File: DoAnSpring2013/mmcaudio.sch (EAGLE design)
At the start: 85 parts, among them IC1 TL082, IC2 TL082, IC3 LM1117, IC4 TL082, IC5 TL082, U1 DAC0808LCN, U2 TEA2025B, X1 HD44780LCD-1602

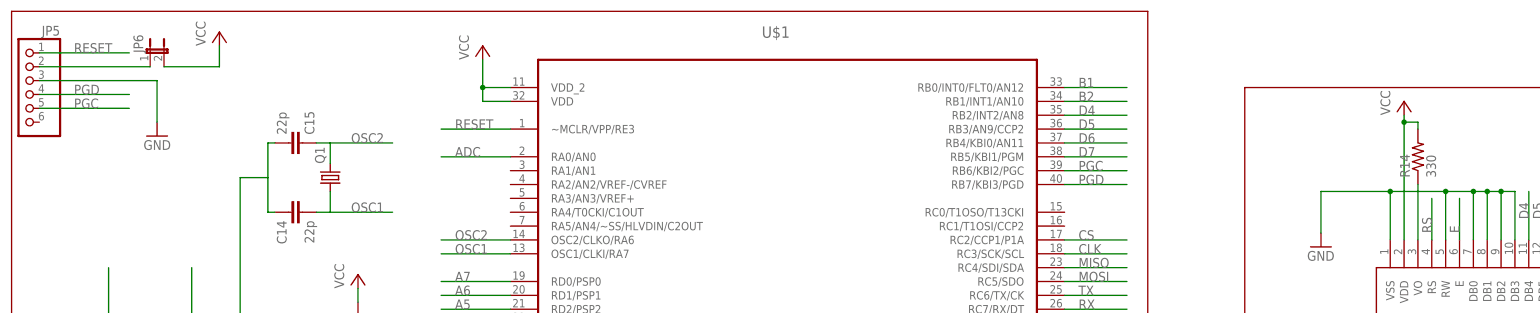
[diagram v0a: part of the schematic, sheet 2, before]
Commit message: routing failed 12:56SA 20131105
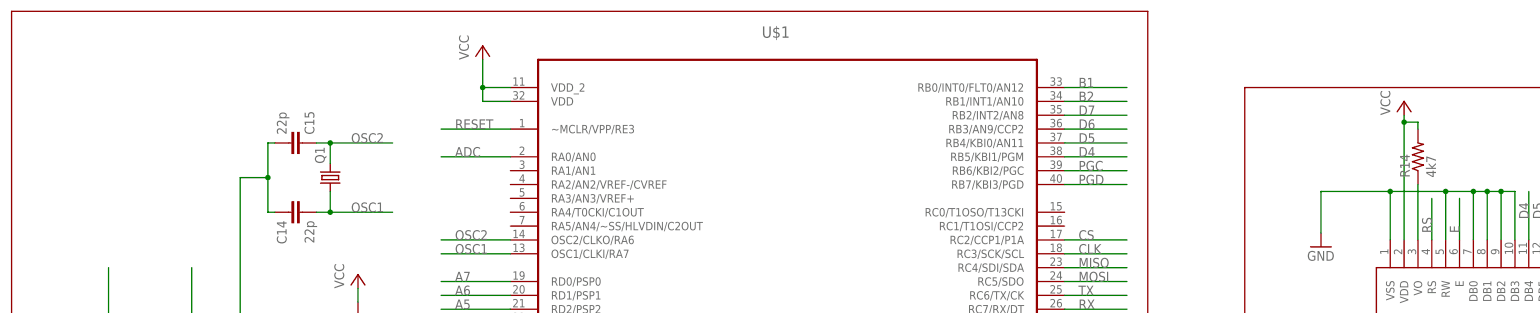
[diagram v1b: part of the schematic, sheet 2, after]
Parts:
- removed JP7: SPEAKER, datle-conn:PINHD-1X20.5"
- removed JP8: (no value), datle-conn:PINHD-1X1
- JP5: value (none) -> SPEAKER; device datle-conn:PINHD-1X6 -> datle-conn:PINHD-1X20.5"
- JP6: device datle-conn:JP1E -> datle-conn:PINHD-1X1
- R14: value 330 -> 4k7
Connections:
- removed net N$42: JP5.2, JP6.1
- net D4: now also U$1.RB5/KBI1/PGM; no longer U$1.RB2/INT2/AN8
- net D5: now also U$1.RB4/KBI0/AN11; no longer U$1.RB3/AN9/CCP2
- net D6: now also U$1.RB3/AN9/CCP2; no longer U$1.RB4/KBI0/AN11
- net D7: now also U$1.RB2/INT2/AN8; no longer U$1.RB5/KBI1/PGM
- net GND: now also JP5.2; no longer JP5.3, JP7.2
- net N$21: now also JP6.1; no longer JP8.1
- net N$25: now also JP5.1; no longer JP7.1
- net PGC: no longer JP5.5
- net PGD: no longer JP5.4
- net RESET: no longer JP5.1
- net VCC: no longer JP6.2
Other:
- moved on the sheet: R23

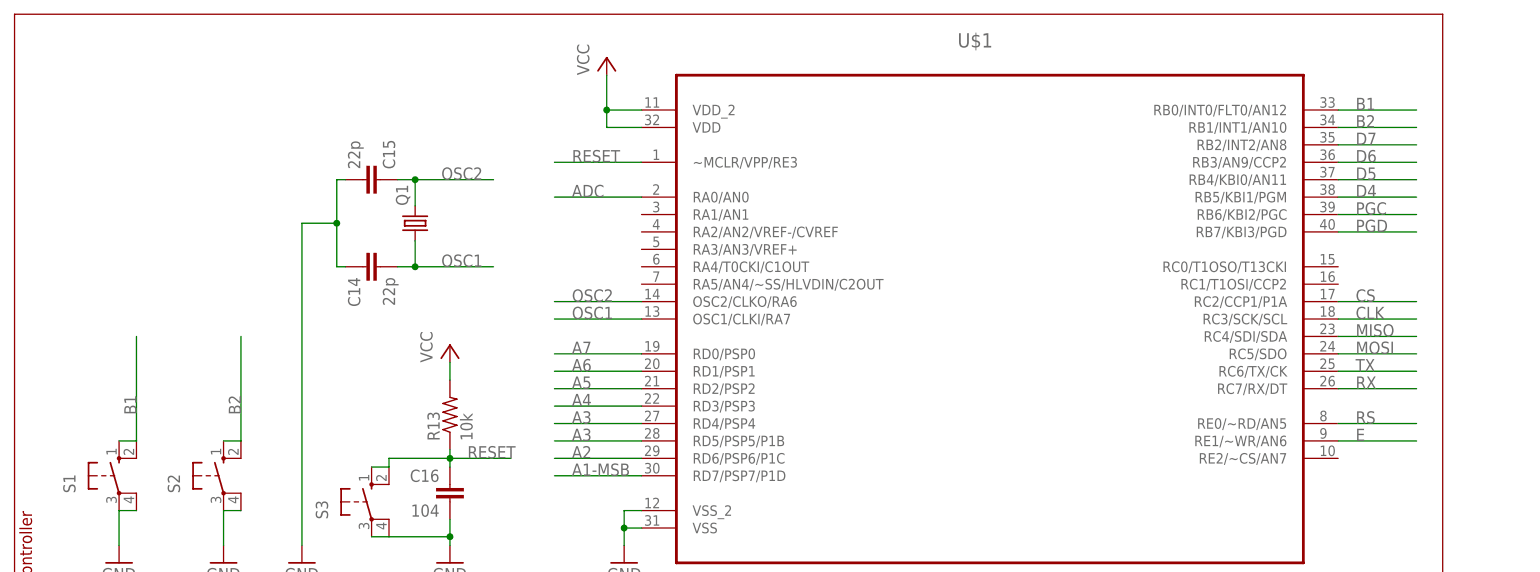
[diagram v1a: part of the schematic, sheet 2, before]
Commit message: route done 1
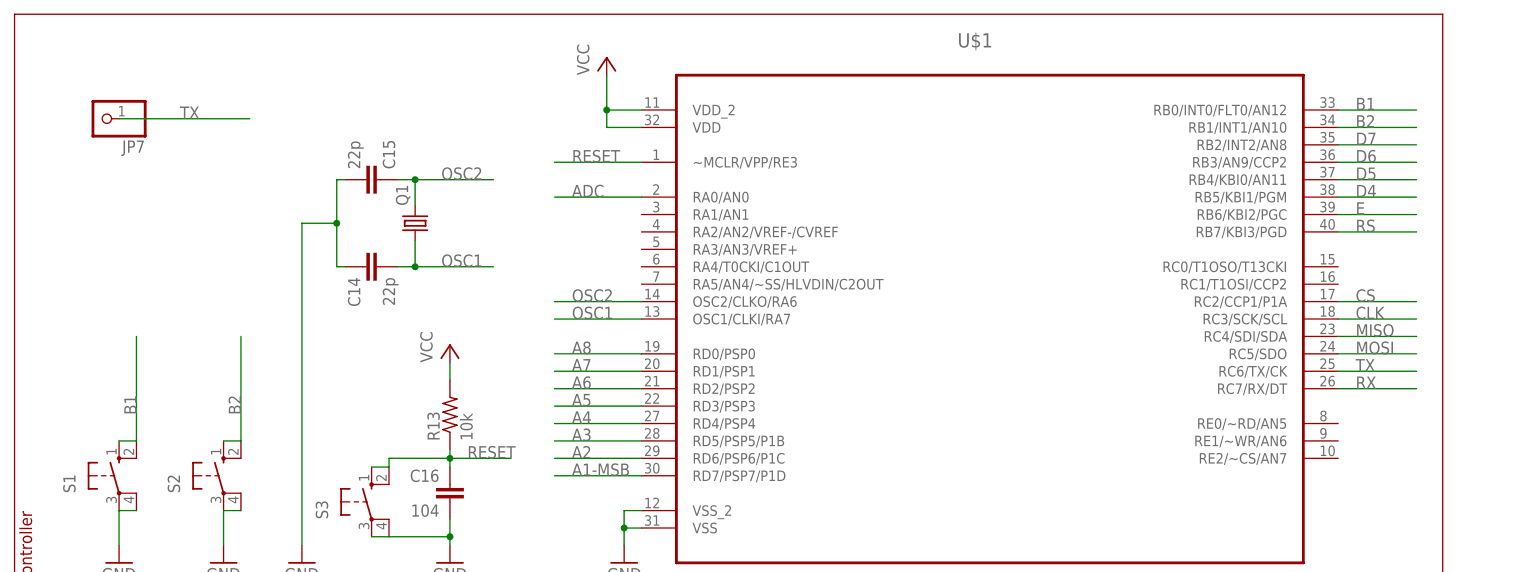
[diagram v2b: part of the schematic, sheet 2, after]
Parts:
- added JP7: (no value), datle-conn:PINHD-1X1
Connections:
- removed net N$35: U$1.RD5/PSP5/P1B
- removed net PGC: U$1.RB6/KBI2/PGC
- removed net PGD: U$1.RB7/KBI3/PGD
- net A3: now also U$1.RD5/PSP5/P1B; no longer U$1.RD4/PSP4
- net A4: now also U$1.RD4/PSP4; no longer U$1.RD3/PSP3
- net A5: now also U$1.RD3/PSP3; no longer U$1.RD2/PSP2
- net A6: now also U$1.RD2/PSP2; no longer U$1.RD1/PSP1
- net A7: now also U$1.RD1/PSP1; no longer U$1.RD0/PSP0
- net A8: now also U$1.RD0/PSP0
- net E: now also U$1.RB6/KBI2/PGC; no longer U$1.RE1/~WR/AN6
- net RS: now also U$1.RB7/KBI3/PGD; no longer U$1.RE0/~RD/AN5
- net TX: now also JP7.1
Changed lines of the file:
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@@
 <setting verticaltext="up"/>
 </settings>
-<grid distance="0.1" unitdist="inch" unit="inch" style="lines" multiple="1" display="no" altdistance="0.01" altunitdist="inch" altunit="mil"/>
+<grid distance="50" unitdist="mil" unit="mil" style="lines" multiple="1" display="yes" altdistance="0.01" altunitdist="inch" altunit="mil"/>
 <layers>
 <layer number="1" name="Top" color="4" fill="1" visible="no" active="no"/>
@@
 <part name="GND1" library="supply1" deviceset="GND" device=""/>
 <part name="GND19" library="supply1" deviceset="GND" device=""/>
+<part name="JP7" library="datle-conn" deviceset="PINHD-1X1" device=""/>
 </parts>
 <sheets>
@@
 <instance part="GND1" gate="1" x="66.04" y="99.06"/>
 <instance part="GND19" gate="1" x="81.28" y="99.06"/>
+<instance part="JP7" gate="G$1" x="63.5" y="163.83" rot="R180"/>
 </instances>
 <busses>
@@
 </segment>
 <segment>
-<pinref part="U$1" gate="A" pin="RE0/~RD/AN5"/>
-<wire x1="243.84" y1="119.38" x2="255.27" y2="119.38" width="0.1524" layer="91"/>
-<label x="246.38" y="119.38" size="1.778" layer="95"/>
+<pinref part="U$1" gate="A" pin="RB7/KBI3/PGD"/>
+<wire x1="243.84" y1="147.32" x2="255.27" y2="147.32" width="0.1524" layer="91"/>
+<label x="246.38" y="147.32" size="1.778" layer="95"/>
 </segment>
 </net>
@@
 <label x="316.23" y="138.43" size="1.778" layer="95" rot="R90"/>
 </segment>
-<segment>
-<pinref part="U$1" gate="A" pin="RE1/~WR/AN6"/>
-<wire x1="243.84" y1="116.84" x2="255.27" y2="116.84" width="0.1524" layer="91"/>
-<label x="246.38" y="116.84" size="1.778" layer="95"/>
-</segment>
-</net>
-<net name="PGD" class="0">
-<segment>
-<pinref part="U$1" gate="A" pin="RB7/KBI3/PGD"/>
-<wire x1="243.84" y1="147.32" x2="255.27" y2="147.32" width="0.1524" layer="91"/>
-<label x="246.38" y="147.32" size="1.778" layer="95"/>
-</segment>
-</net>
-<net name="PGC" class="0">
 <segment>
 <pinref part="U$1" gate="A" pin="RB6/KBI2/PGC"/>
@@
 <label x="246.38" y="127" size="1.778" layer="95"/>
 </segment>
+<segment>
+<pinref part="JP7" gate="G$1" pin="1"/>
+<wire x1="66.04" y1="163.83" x2="85.09" y2="163.83" width="0.1524" layer="91"/>
+<label x="74.93" y="163.83" size="1.778" layer="95"/>
+</segment>
 </net>
 <net name="RX" class="0">
@@
 </segment>
 </net>
-<net name="A3" class="0">
+<net name="A4" class="0">
 <segment>
 <pinref part="U$1" gate="A" pin="RD4/PSP4"/>
-<wire x1="129.54" y1="119.38" x2="142.24" y2="119.38" width="0.1524" layer="91"/>
-<label x="132.08" y="116.84" size="1.778" layer="95"/>
+<wire x1="142.24" y1="119.38" x2="129.54" y2="119.38" width="0.1524" layer="91"/>
 <label x="132.08" y="119.38" size="1.778" layer="95"/>
 </segment>
 </net>
-<net name="A4" class="0">
+<net name="A5" class="0">
 <segment>
 <pinref part="U$1" gate="A" pin="RD3/PSP3"/>
@@
 </segment>
 </net>
-<net name="A5" class="0">
+<net name="A6" class="0">
 <segment>
 <pinref part="U$1" gate="A" pin="RD2/PSP2"/>
@@
 </segment>
 </net>
-<net name="A6" class="0">
+<net name="A7" class="0">
 <segment>
 <pinref part="U$1" gate="A" pin="RD1/PSP1"/>
@@
 </segment>
 </net>
-<net name="A7" class="0">
-<segment>
-<pinref part="U$1" gate="A" pin="RD0/PSP0"/>
-<wire x1="142.24" y1="129.54" x2="129.54" y2="129.54" width="0.1524" layer="91"/>
-<label x="132.08" y="129.54" size="1.778" layer="95"/>
-</segment>
-</net>
-<net name="N$35" class="0">
+<net name="A3" class="0">
 <segment>
 <pinref part="U$1" gate="A" pin="RD5/PSP5/P1B"/>
 <wire x1="142.24" y1="116.84" x2="129.54" y2="116.84" width="0.1524" layer="91"/>
+<label x="132.08" y="116.84" size="1.778" layer="95"/>
 </segment>
 </net>
@@
 </segment>
 </net>
+<net name="A8" class="0">
+<segment>
+<pinref part="U$1" gate="A" pin="RD0/PSP0"/>
+<wire x1="142.24" y1="129.54" x2="129.54" y2="129.54" width="0.1524" layer="91"/>
+<label x="132.08" y="129.54" size="1.778" layer="95"/>
+</segment>
+</net>

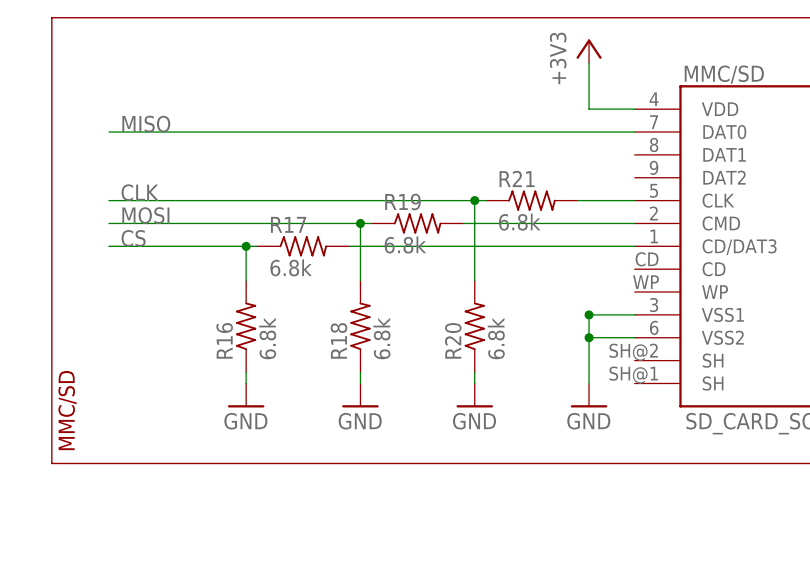
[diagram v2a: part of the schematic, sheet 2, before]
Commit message: clean the fault
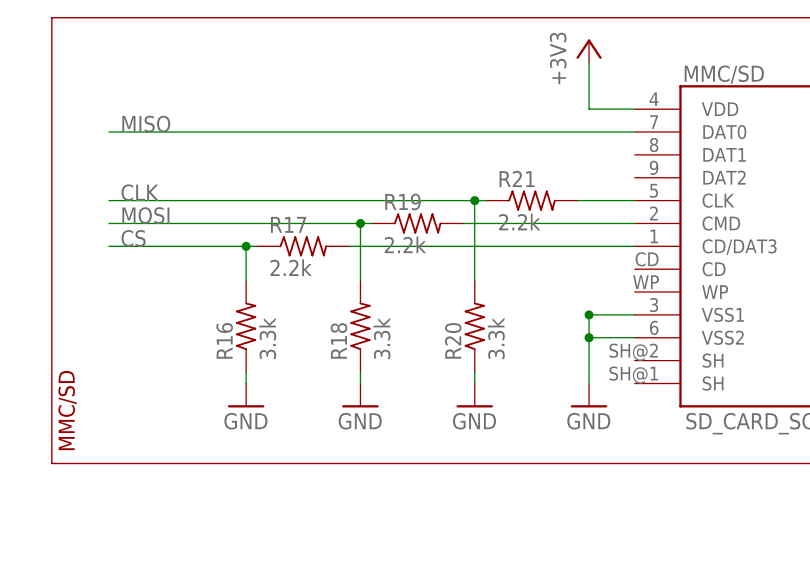
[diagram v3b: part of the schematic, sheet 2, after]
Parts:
- R16, R18, R20: value 6.8k -> 3.3k
- R17, R19, R21: value 6.8k -> 2.2k
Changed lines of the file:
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@@
 <setting verticaltext="up"/>
 </settings>
-<grid distance="50" unitdist="mil" unit="mil" style="lines" multiple="1" display="yes" altdistance="0.01" altunitdist="inch" altunit="mil"/>
+<grid distance="0.1" unitdist="inch" unit="inch" style="lines" multiple="1" display="no" altdistance="0.01" altunitdist="inch" altunit="inch"/>
 <layers>
 <layer number="1" name="Top" color="4" fill="1" visible="no" active="no"/>
@@
 <part name="MMC/SD" library="datle-discrete" deviceset="SD_CARD_SOCKET" device="4UCON"/>
 <part name="GND28" library="supply1" deviceset="GND" device=""/>
-<part name="R21" library="datle-discrete" deviceset="R-US_" device="0207/10" value="6.8k"/>
-<part name="R19" library="datle-discrete" deviceset="R-US_" device="0207/10" value="6.8k"/>
-<part name="R17" library="datle-discrete" deviceset="R-US_" device="0207/10" value="6.8k"/>
-<part name="R16" library="datle-discrete" deviceset="R-US_" device="0207/10" value="6.8k"/>
-<part name="R18" library="datle-discrete" deviceset="R-US_" device="0207/10" value="6.8k"/>
-<part name="R20" library="datle-discrete" deviceset="R-US_" device="0207/10" value="6.8k"/>
+<part name="R21" library="datle-discrete" deviceset="R-US_" device="0207/10" value="2.2k"/>
+<part name="R19" library="datle-discrete" deviceset="R-US_" device="0207/10" value="2.2k"/>
+<part name="R17" library="datle-discrete" deviceset="R-US_" device="0207/10" value="2.2k"/>
+<part name="R16" library="datle-discrete" deviceset="R-US_" device="0207/10" value="3.3k"/>
+<part name="R18" library="datle-discrete" deviceset="R-US_" device="0207/10" value="3.3k"/>
+<part name="R20" library="datle-discrete" deviceset="R-US_" device="0207/10" value="3.3k"/>
 <part name="GND29" library="supply1" deviceset="GND" device=""/>
 <part name="GND30" library="supply1" deviceset="GND" device=""/>
